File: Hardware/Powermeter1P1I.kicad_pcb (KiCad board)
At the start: 4 copper layers, 50 x 62 mm, 76 parts, among them IC1 CH32V003F4U6, IC3 RY8310, J1 Conn_01x04_Pin, J2 Conn_01x04_Pin, J3 Conn_01x02_Socket, J4 Conn_01x01_Socket, J5 Conn_01x01_Socket, J6 Conn_01x01_Socket, J7 Conn_01x01_Socket, J8 Conn_01x02_Socket, J9 TagConnect, Q2 AO3401A, U1 MAX485, U2 BL0942_C2909509, U3 XC6206P332MR, U5 TEA1-0505

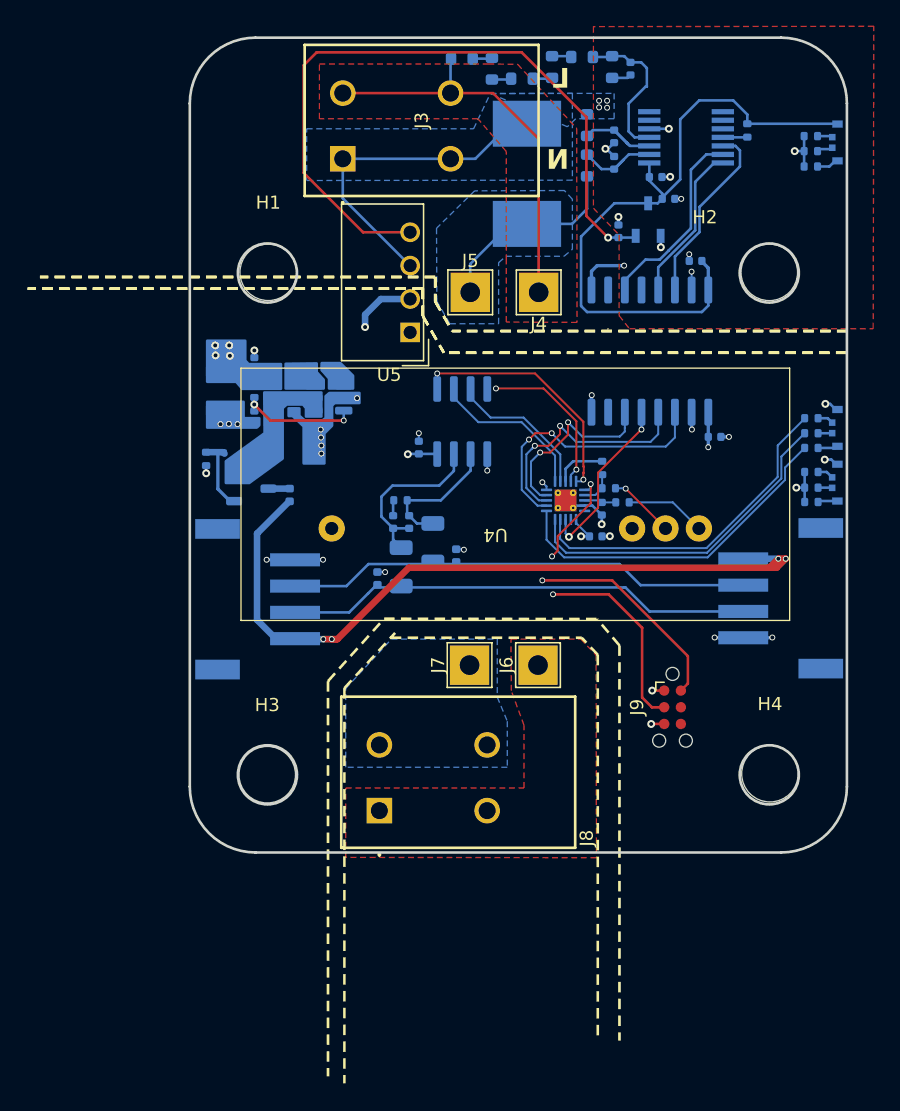
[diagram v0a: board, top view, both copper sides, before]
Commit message: add all
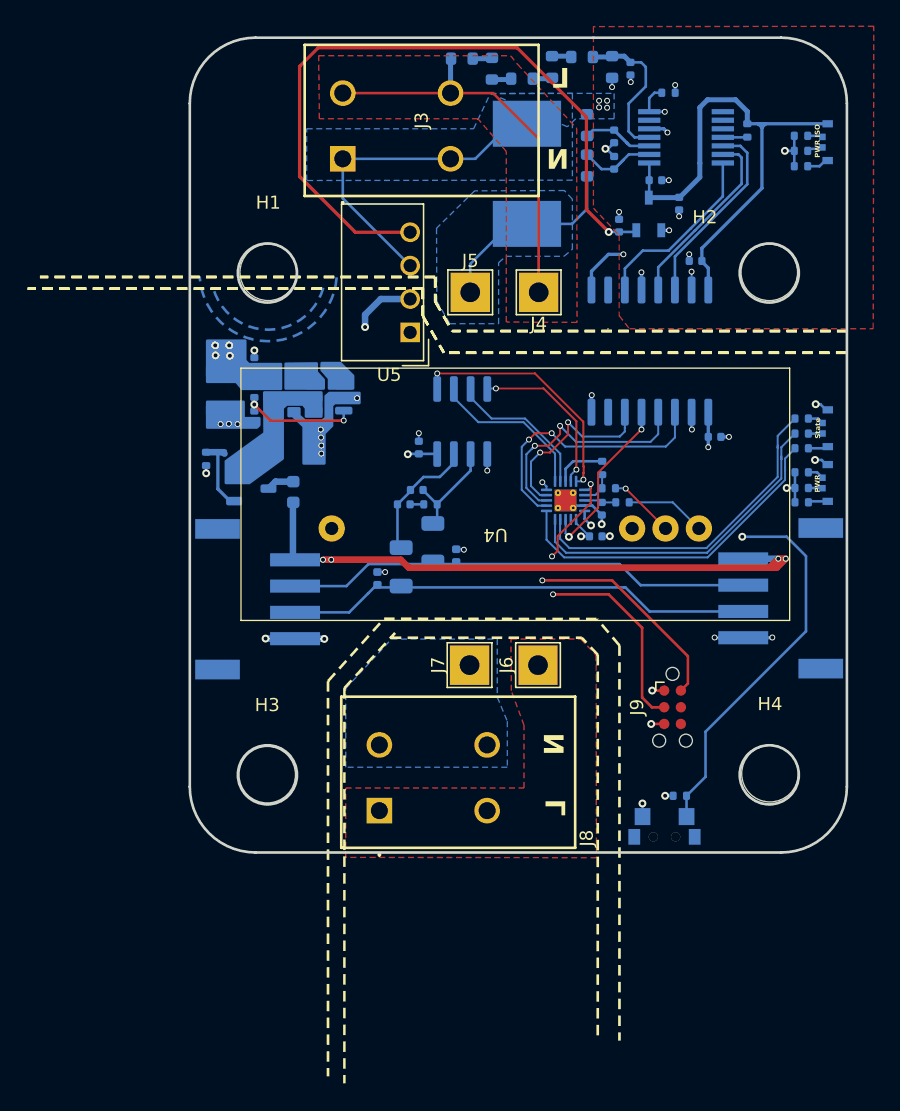
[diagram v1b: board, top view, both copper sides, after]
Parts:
- added R17: 4k7, Resistor_SMD:R_0402_1005Metric, B.Cu at (150.1, 69.1)
- added R27: 4k7, Resistor_SMD:R_0402_1005Metric, B.Cu at (150.9, 122.6)
- added SW1: SW_Push, LCSC:SW-SMD_TS24CA, B.Cu at (149.8, 125.0)
- F2: footprint Fuse:Fuse_0402_1005Metric -> Fuse:Fuse_0603_1608Metric
- moved R5 2.50 mm to (130.9, 99.3), turned to 0 degrees
- moved R3 2.30 mm to (132.0, 100.4)
- moved C2 1.57 mm to (129.9, 100.4), turned to 0 degrees
- moved C19 0.88 mm to (150.9, 77.5), turned to -90 degrees
- moved R16 0.75 mm to (160.1, 74.7)
- moved D3 0.75 mm to (162.0, 72.9)
- moved R15 0.75 mm to (160.1, 73.5)
- moved R7 0.75 mm to (160.1, 72.4)
- moved D6 0.74 mm to (162.0, 94.6)
- moved R13 0.74 mm to (160.2, 99.2)
- moved R14 0.74 mm to (160.2, 100.3)
- moved R18 0.74 mm to (160.2, 96.2)
- moved R19 0.74 mm to (160.2, 95.0)
- moved R20 0.74 mm to (160.2, 93.9)
- moved R9 0.74 mm to (160.2, 98.0)
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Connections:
- C7 pad 2: Net-(C7-Pad2) -> GND1
- IC1 pad 5: unconnected-(IC1-PD0-Pad5) -> Button
- J2 pad 1: VCC -> GND
- J2 pad 4: GND -> VCC
- R21 pad 2: Net-(C7-Pad2) -> GND1
- U2 pad 13: MISO_ISO -> MOSI_ISO
- U2 pad 14: MOSI_ISO -> MISO_ISO
- U2 pad 7: unconnected-(U2-A2_NCS-Pad7) -> CS_ISO
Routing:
- net Button: track 0.00 -> 43.7 mm, vias 0 -> 2
- net CS_ISO: track 0.00 -> 17.7 mm, vias 0 -> 2
- net +3.3V: track 49.8 -> 40.0 mm
- net VCC: track 61.6 -> 52.0 mm
- net Net-(U1-B): track 13.3 -> 9.74 mm
- net GND: track 38.3 -> 41.0 mm, vias 25 -> 26
- net Net-(U1-A): track 10.3 -> 8.01 mm
- net MOSI_ISO: track 12.9 -> 15.1 mm
- net GND1: track 40.1 -> 42.2 mm, vias 14 -> 17
- net Net-(C7-Pad2): track 1.49 -> 0.00 mm
- net MISO_ISO: track 14.8 -> 13.9 mm
- net SCLK_ISO: track 15.0 -> 15.7 mm
- net RS485_TX: track 11.9 -> 12.6 mm
- net Net-(U3-Vin): track 54.1 -> 54.7 mm
- net +5V: track 23.7 -> 24.3 mm, vias 11 -> 12
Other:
- board text added: "PWR"
- board text added: "PWR ISO"
- board text added: "State"
